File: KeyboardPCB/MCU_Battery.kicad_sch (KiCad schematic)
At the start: 41 parts, among them Q1 CSD17527Q5A, Q2 CSD17527Q5A, U1 ATmega32U4-M, U2 TPS61236PRWLT, U3 BQ297xy, U4 BQ24193RGER, Y1 ECS-160-7-33B-CKL-TR

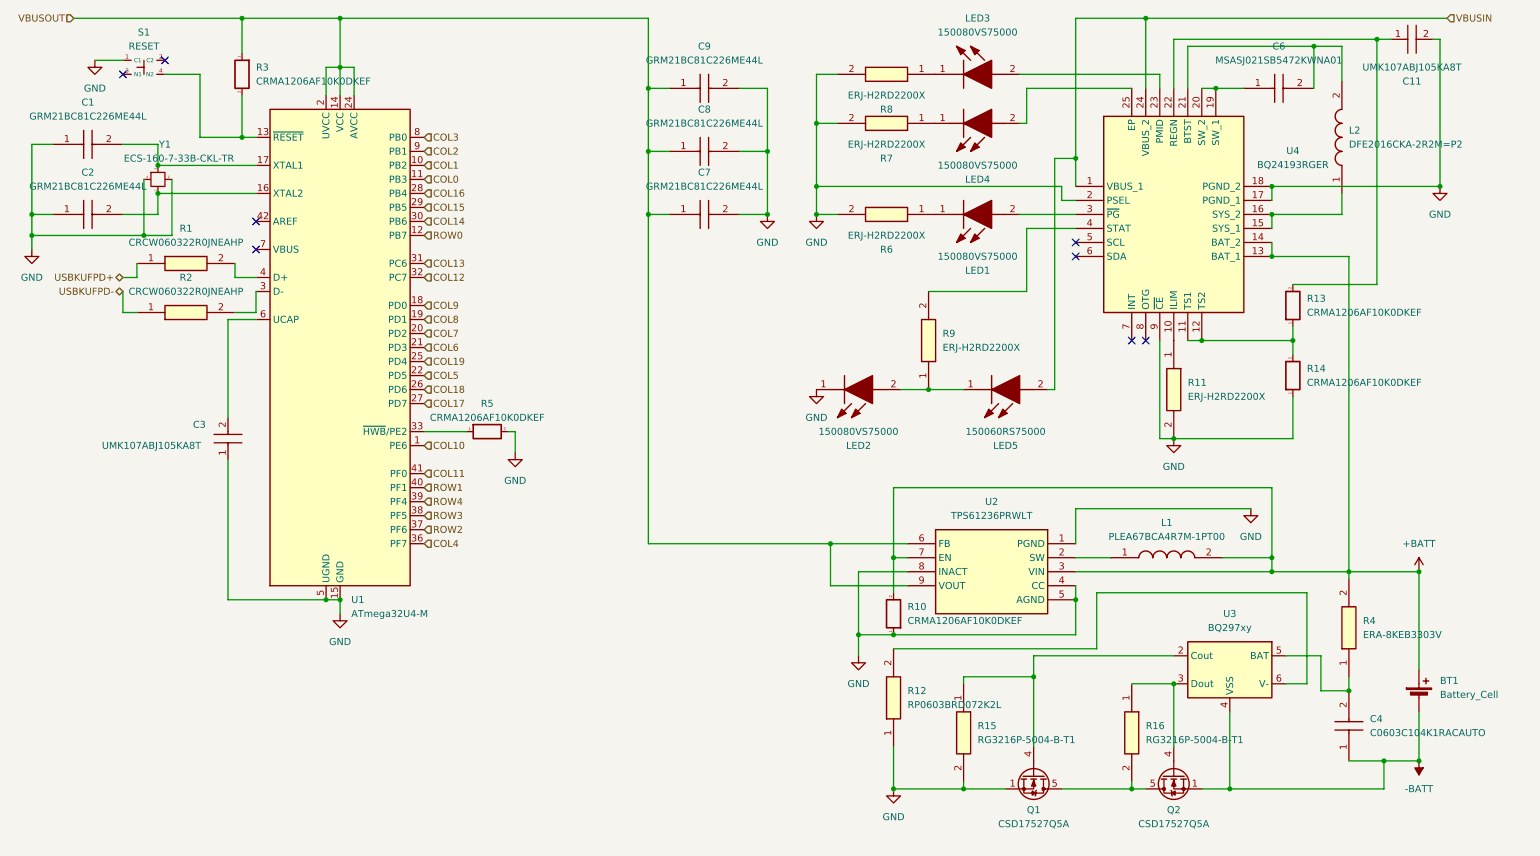
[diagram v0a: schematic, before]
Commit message: Began routing PCB
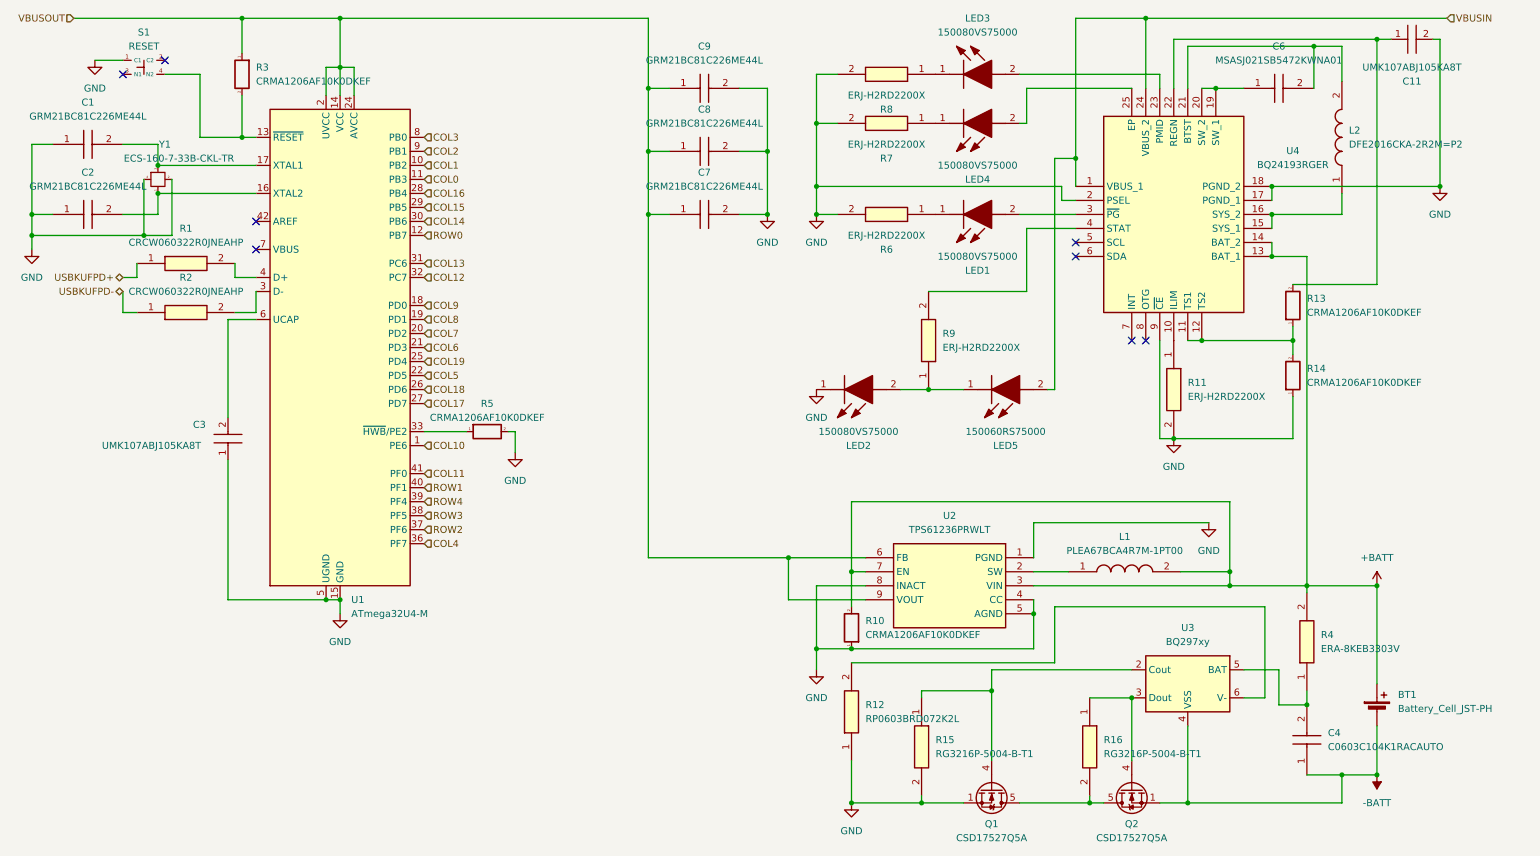
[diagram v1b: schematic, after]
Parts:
- removed BT1: Battery_Cell, symbol Device:Battery_Cell
- added BT1: Battery_Cell_JST-PH, Connector_JST:JST_PH_B2B-PH-K_1x02_P2.00mm_Vertical, symbol keyboard_syms:Battery_Cell_JST-PH
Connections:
- net +BATT: now also BT1.1 (+)
- net -BATT: now also BT1.2 (-)
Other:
- moved on the sheet: C4, L1, Q1, Q2, R10, R12, R15, R16, R4, U2, U3
